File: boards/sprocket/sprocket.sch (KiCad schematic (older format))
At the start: 35 parts, among them J1 SPROCKET-CONN, J4 Conn_01x04_MountingPin, J5 Conn_01x04_MountingPin, J6 Conn_01x04_MountingPin, J7 Conn_01x04_MountingPin, Q1 NX7002BKR, SW1 SW_Push, SW2 SW_Push, U1 STM32G031G8U6, U2 AP2210N-3.3TRG1

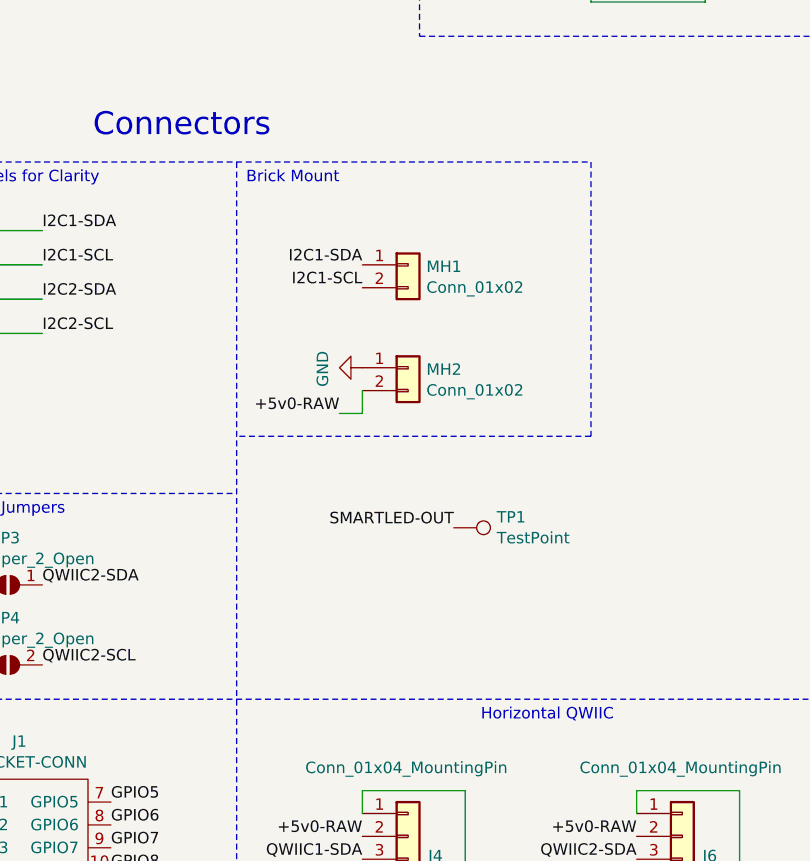
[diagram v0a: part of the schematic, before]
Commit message: Add recent projects
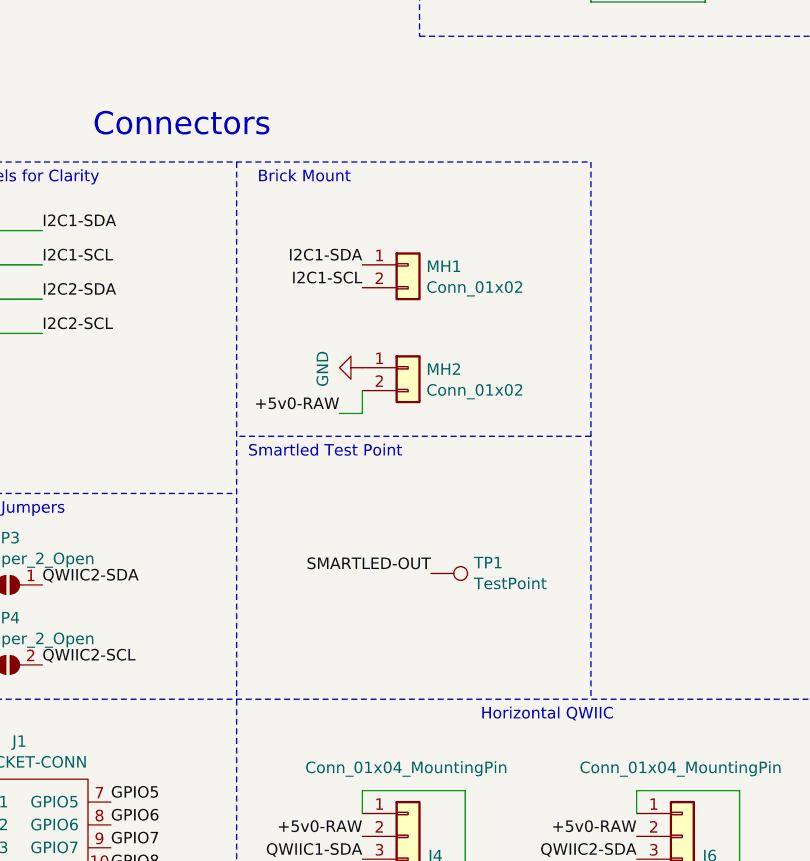
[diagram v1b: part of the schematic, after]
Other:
- note added: "Smartled Test Point"
- moved on the sheet: TP1
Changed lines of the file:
@@
 Wire Wire Line
 	2900 3750 2900 3650
-Text Notes 2800 2750 2    50   ~ 0
+Text Notes 2850 2750 2    50   ~ 0
 Brick Mount
 Wire Notes Line
@@
 	1500 3400 1200 3400
 Wire Notes Line
-	3900 2650 3900 3850
-Wire Notes Line
 	500  4100 2350 4100
 Wire Notes Line
@@
 L Connector:TestPoint TP1
 U 1 1 6047197A
-P 3300 4250
-F 0 "TP1" V 3254 4438 50  0000 L CNN
-F 1 "TestPoint" V 3345 4438 50  0000 L CNN
-F 2 "TestPoint:TestPoint_Pad_D1.5mm" H 3500 4250 50  0001 C CNN
-F 3 "~" H 3500 4250 50  0001 C CNN
-	1    3300 4250
+P 3200 4450
+F 0 "TP1" V 3154 4638 50  0000 L CNN
+F 1 "TestPoint" V 3245 4638 50  0000 L CNN
+F 2 "TestPoint:TestPoint_Pad_D1.5mm" H 3400 4450 50  0001 C CNN
+F 3 "~" H 3400 4450 50  0001 C CNN
+	1    3200 4450
 	0    1    1    0
 $EndComp
-Text Label 3300 4250 2    50   ~ 0
+Text Label 3200 4450 2    50   ~ 0
 SMARTLED-OUT
+Wire Notes Line
+	3900 2650 3900 5000
+Text Notes 2400 3950 0    50   ~ 0
+Smartled Test Point
 $EndSCHEMATC
